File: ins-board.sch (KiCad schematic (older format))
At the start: 58 parts, among them P1 PWR, U2 STM32F415RGT6, U4 MAX3051, X1 CRYSTAL 16MHz 10ppm

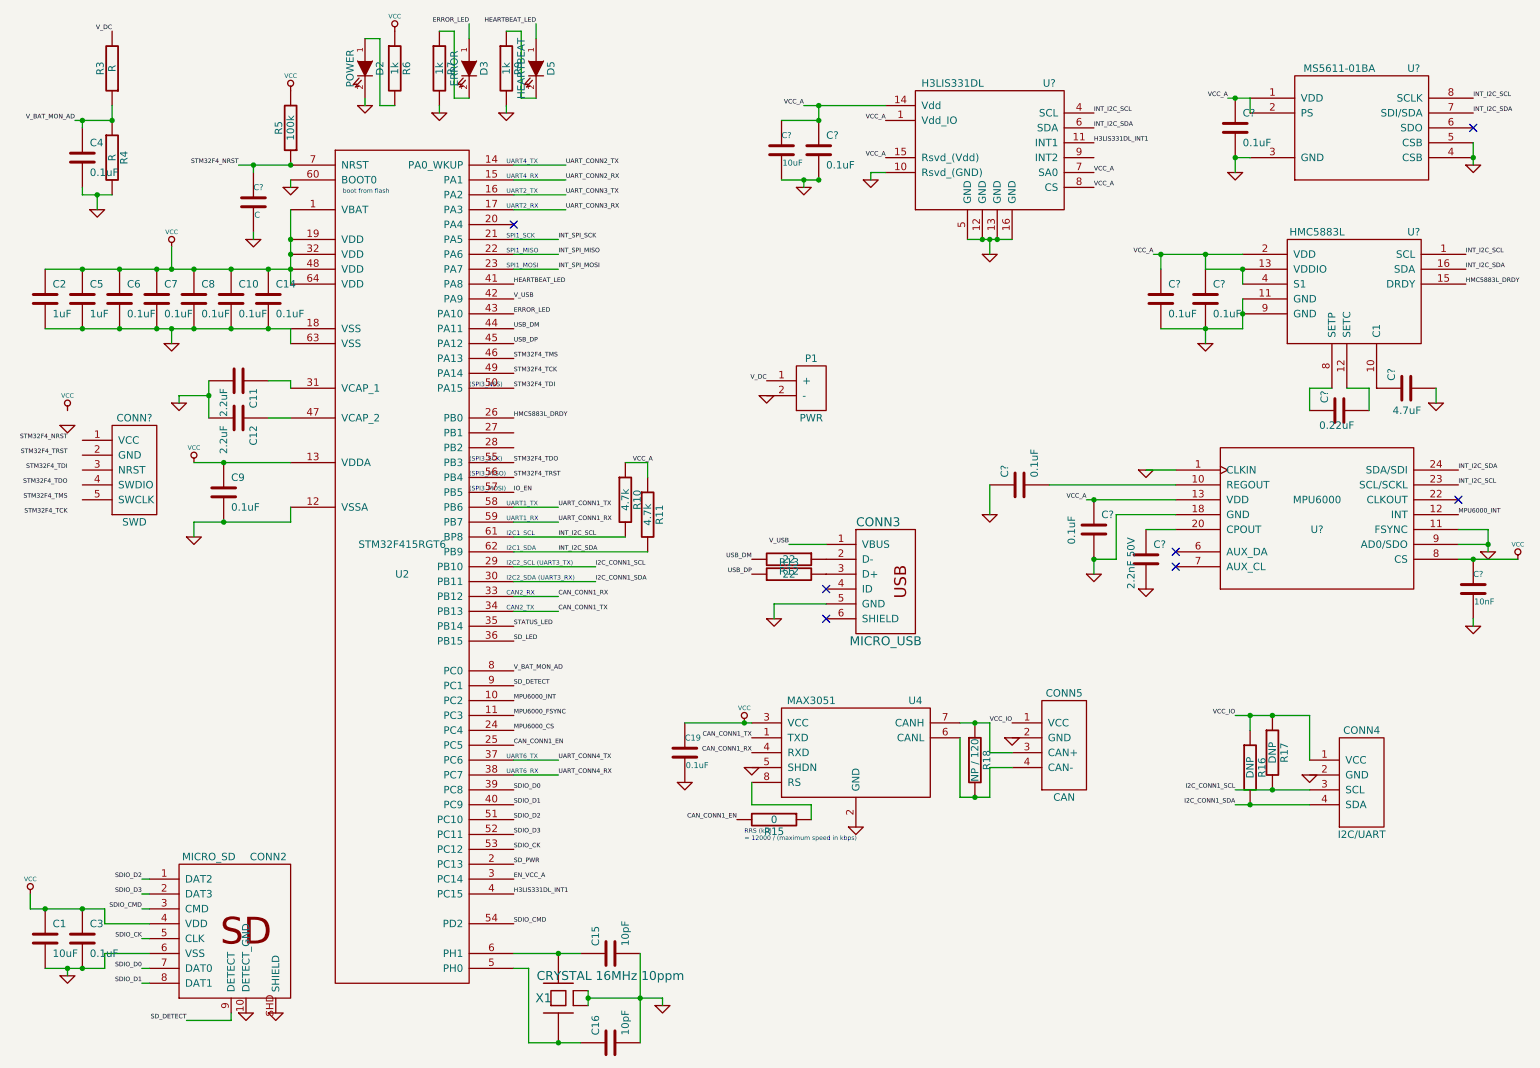
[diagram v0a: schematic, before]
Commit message: schematics
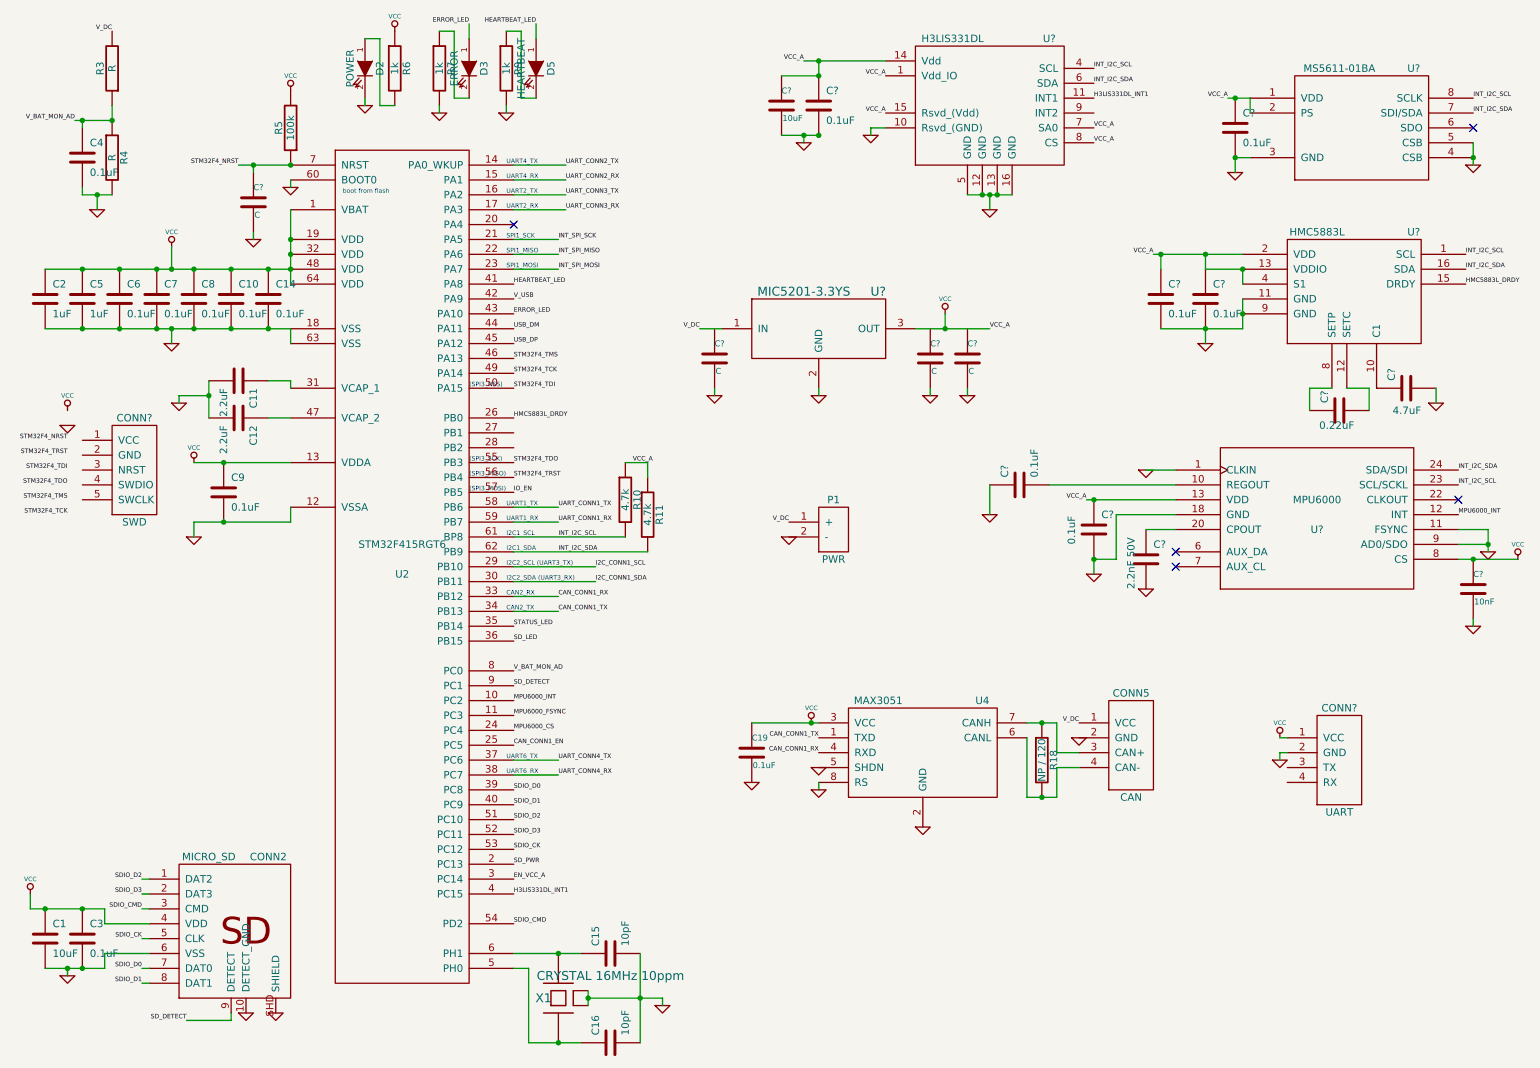
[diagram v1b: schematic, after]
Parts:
- removed CONN3: MICRO_USB, symbol MICRO_USB
- removed CONN4: I2C/UART, MODULE, symbol I2C
- removed R12, R13: 22, symbol R
- removed R15: 0, symbol R
- removed R16, R17: DNP, symbol R
- added C? (x3): C, symbol C
- added CONN?: UART, MODULE, symbol UART
- added U?: MIC5201-3.3YS, symbol MIC5201-3.3YS
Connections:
- net VCC_A is gone; now on net VCC: C?.1, C?.1, C?.1, C?.1, C?.1, C?.1, R10.1, R11.1, U?.1 (VDD), U?.1 (Vdd_IO), U?.13 (VDD), U?.13 (VDDIO), U?.14 (Vdd), U?.15 (Rsvd_(Vdd)), U?.2 (PS), U?.2 (VDD), U?.4 (S1), U?.7 (SA0), U?.8 (CS)
- net VCC_IO is gone; now on net V_DC: CONN5.1 (VCC)
- net GND: now also U4.8 (RS), C?.2, C?.2, C?.2, CONN?.2 (GND), CONN?.MECH (GND), U?.2 (GND)
- net VCC: now also CONN?.1 (VCC), U?.3 (OUT)
- net V_DC: now also U?.1 (IN)
- no-connect marks 7 -> 5
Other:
- note removed: "RRS (kΩ)\n≈ 12000 / (maximum speed in kbps)"
- moved on the sheet: C19, C?, CONN5, P1, R18, U4, U?

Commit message: stm32f042
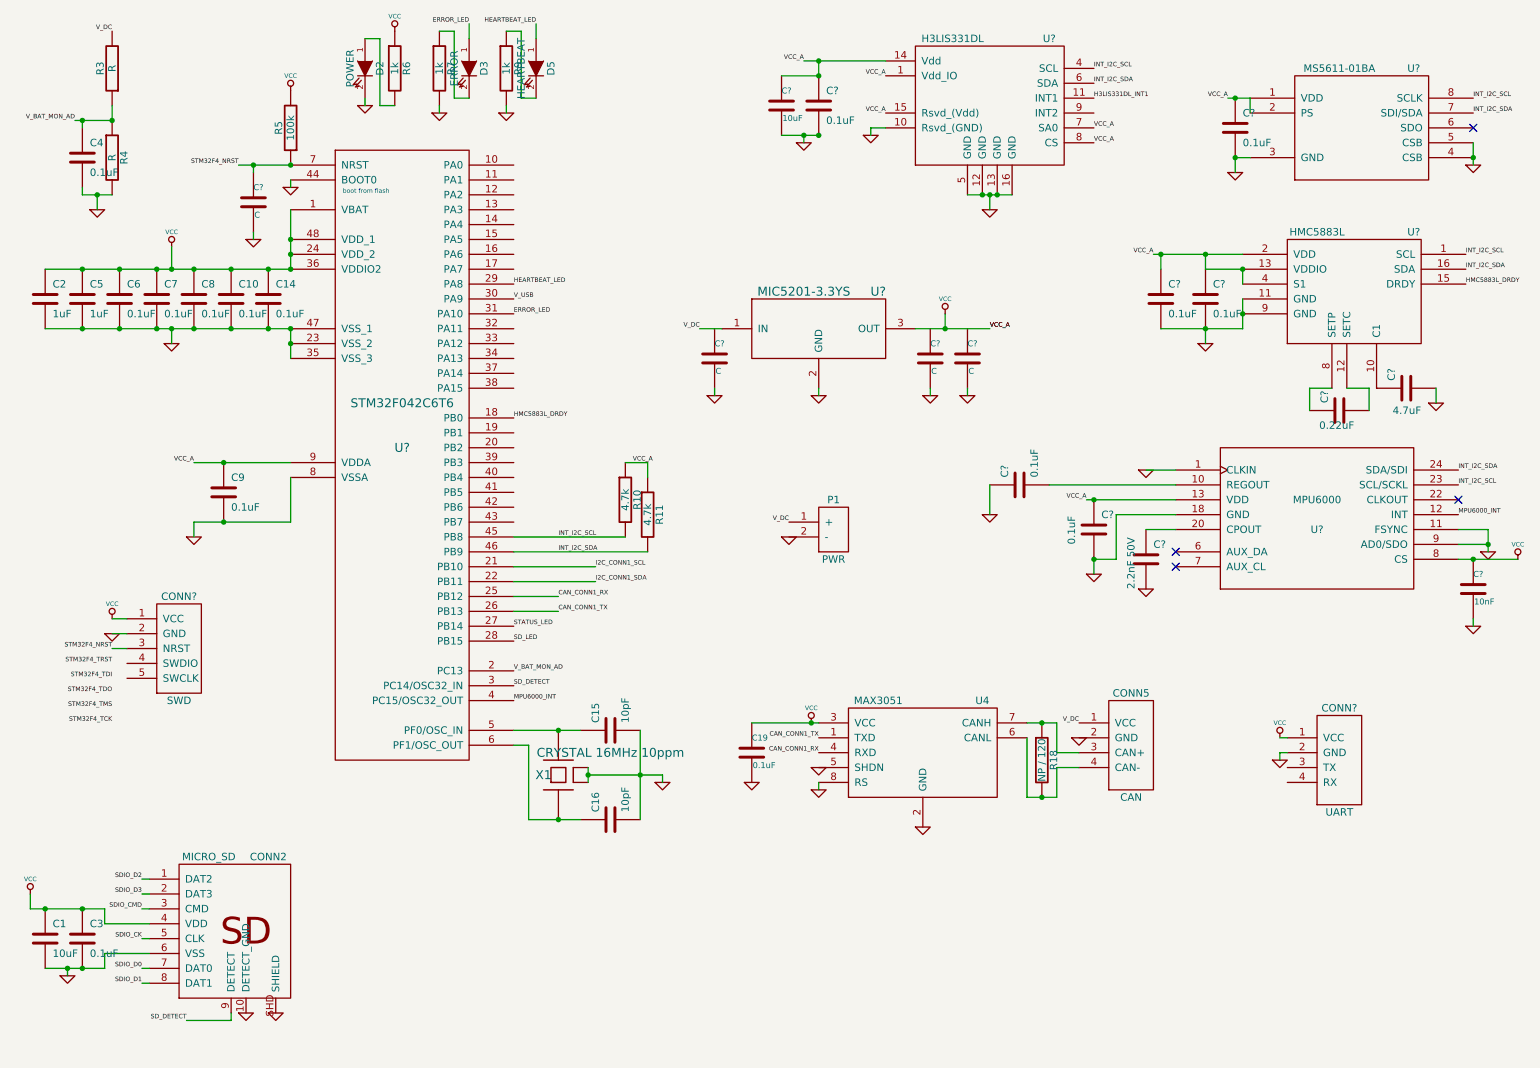
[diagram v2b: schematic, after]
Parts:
- removed C11, C12: 2.2uF, symbol C
- removed U2: STM32F415RGT6, MODULE, symbol STM32F415RGT6
- added U?: STM32F042C6T6, MODULE, symbol STM32F042C6T6
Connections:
- net CAN_CONN1_RX: now also U?.25 (PB12)
- net CAN_CONN1_TX: now also U?.26 (PB13)
- net ERROR_LED: now also U?.31 (PA10)
- net GND: now also CONN?.2 (GND), U?.23 (VSS_2), U?.35 (VSS_3), U?.44 (BOOT0), U?.47 (VSS_1), U?.8 (VSSA)
- net HEARTBEAT_LED: now also U?.29 (PA8)
- net HMC5883L_DRDY: now also U?.18 (PB0)
- net I2C_CONN1_SCL: now also U?.21 (PB10)
- net I2C_CONN1_SDA: now also U?.22 (PB11)
- net INT_I2C_SCL: now also U?.45 (PB8)
- net INT_I2C_SDA: now also U?.46 (PB9)
- net MPU6000_INT: now also U?.4 (PC15/OSC32_OUT)
- net SD_DETECT: now also U?.3 (PC14/OSC32_IN)
- net SD_LED: now also U?.28 (PB15)
- net STATUS_LED: now also U?.27 (PB14)
- net STM32F4_NRST: now also CONN?.3 (NRST), U?.7 (NRST)
- net VCC: now also CONN?.1 (VCC), U?.1 (VBAT), U?.24 (VDD_2), U?.36 (VDDIO2), U?.48 (VDD_1), U?.9 (VDDA)
- net V_BAT_MON_AD: now also U?.2 (PC13)
- net V_USB: now also U?.30 (PA9)
- net at C16.1, X1.1: now also U?.6 (PF1/OSC_OUT)
- net at C15.1, X1.3: now also U?.5 (PF0/OSC_IN)
- no-connect marks 5 -> 4
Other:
- note removed: "(SPI3_MISO)"
- note removed: "(SPI3_MOSI)"
- note removed: "(SPI3_NSS)"
- note removed: "(SPI3_SCK)"
- note removed: "CAN2_RX"
- note removed: "CAN2_TX"
- note removed: "I2C1_SCL"
- note removed: "I2C1_SDA"
- note removed: "I2C2_SCL (UART3_TX)"
- note removed: "I2C2_SDA (UART3_RX)"
- note removed: "SPI1_MISO"
- note removed: "SPI1_MOSI"
- note removed: "SPI1_SCK"
- note removed: "UART1_RX"
- note removed: "UART1_TX"
- note removed: "UART2_RX"
- note removed: "UART2_TX"
- note removed: "UART4_RX"
- note removed: "UART4_TX"
- note removed: "UART6_RX"
- note removed: "UART6_TX"
- moved on the sheet: C15, C16, CONN?, X1
